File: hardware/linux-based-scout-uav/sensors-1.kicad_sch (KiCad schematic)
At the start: 5 parts, among them U5 MPU-6050, U6 AMG8833

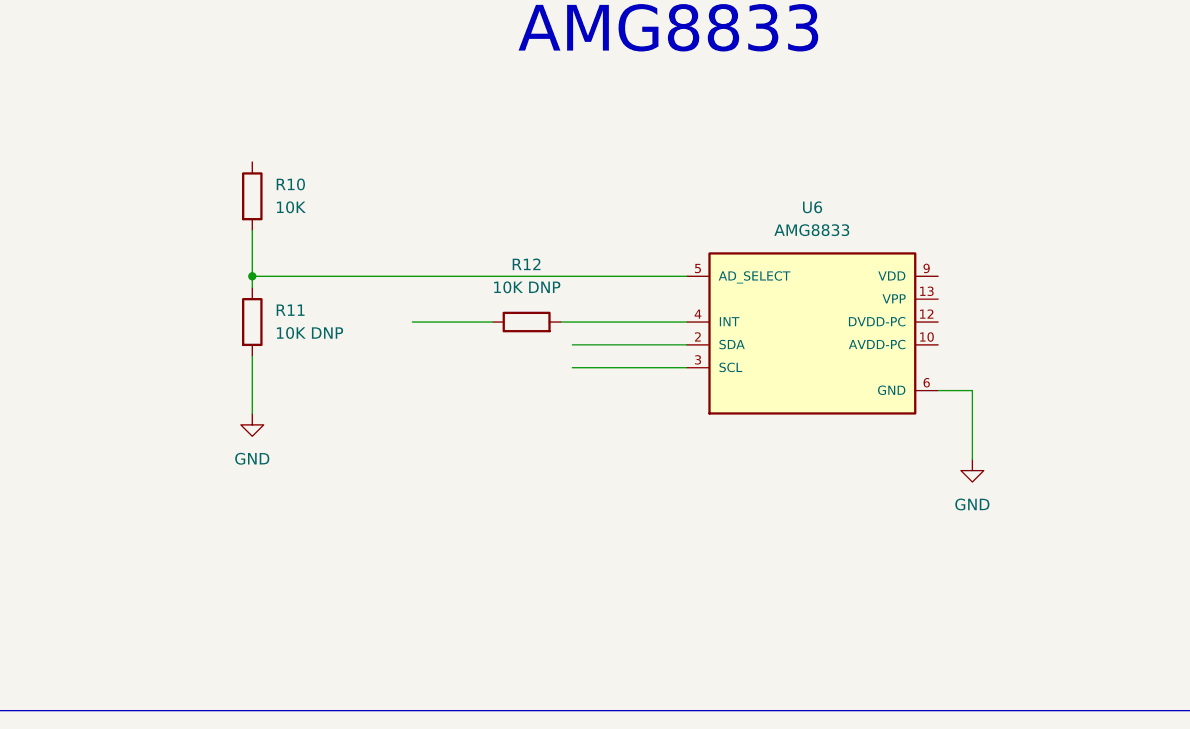
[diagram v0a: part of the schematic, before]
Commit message: Schematic update
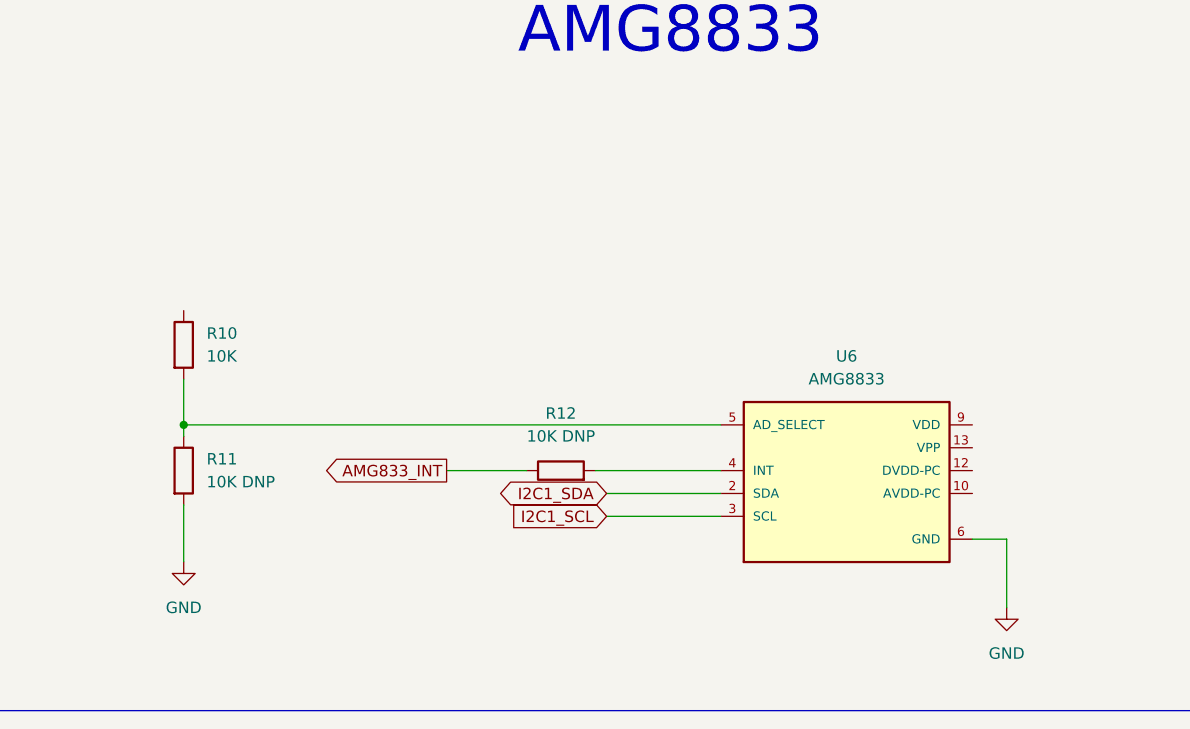
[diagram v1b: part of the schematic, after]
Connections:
- net I2C1_SCL: now also U6.3 (SCL)
- net I2C1_SDA: now also U6.2 (SDA)
- net AMG833_INT: now reaches R12.1
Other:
- moved on the sheet: R10, R11, R12, U6
